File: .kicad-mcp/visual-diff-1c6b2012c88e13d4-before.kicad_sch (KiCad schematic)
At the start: 67 parts, among them J1 USB-C_PWR_IN, J2 USB-C_CPU_PROG, J3 USB-C_UART_BRIDGE, Q1 BSC010NE2LS, Q2 BSC010NE2LS, Q3 BSC010NE2LS, Q4 BSC010NE2LS, Q5 BSC010NE2LS, Q6 BSC010NE2LS, Q7 BSC010NE2LS, Q8 BSC010NE2LS, U1 RP2040, U2 W25Q16JVSSIQ, U3 ISL8117FRZ, U4 ISL8117FRZ, U5 ISL8117FRZ, U6 ISL8117FRZ

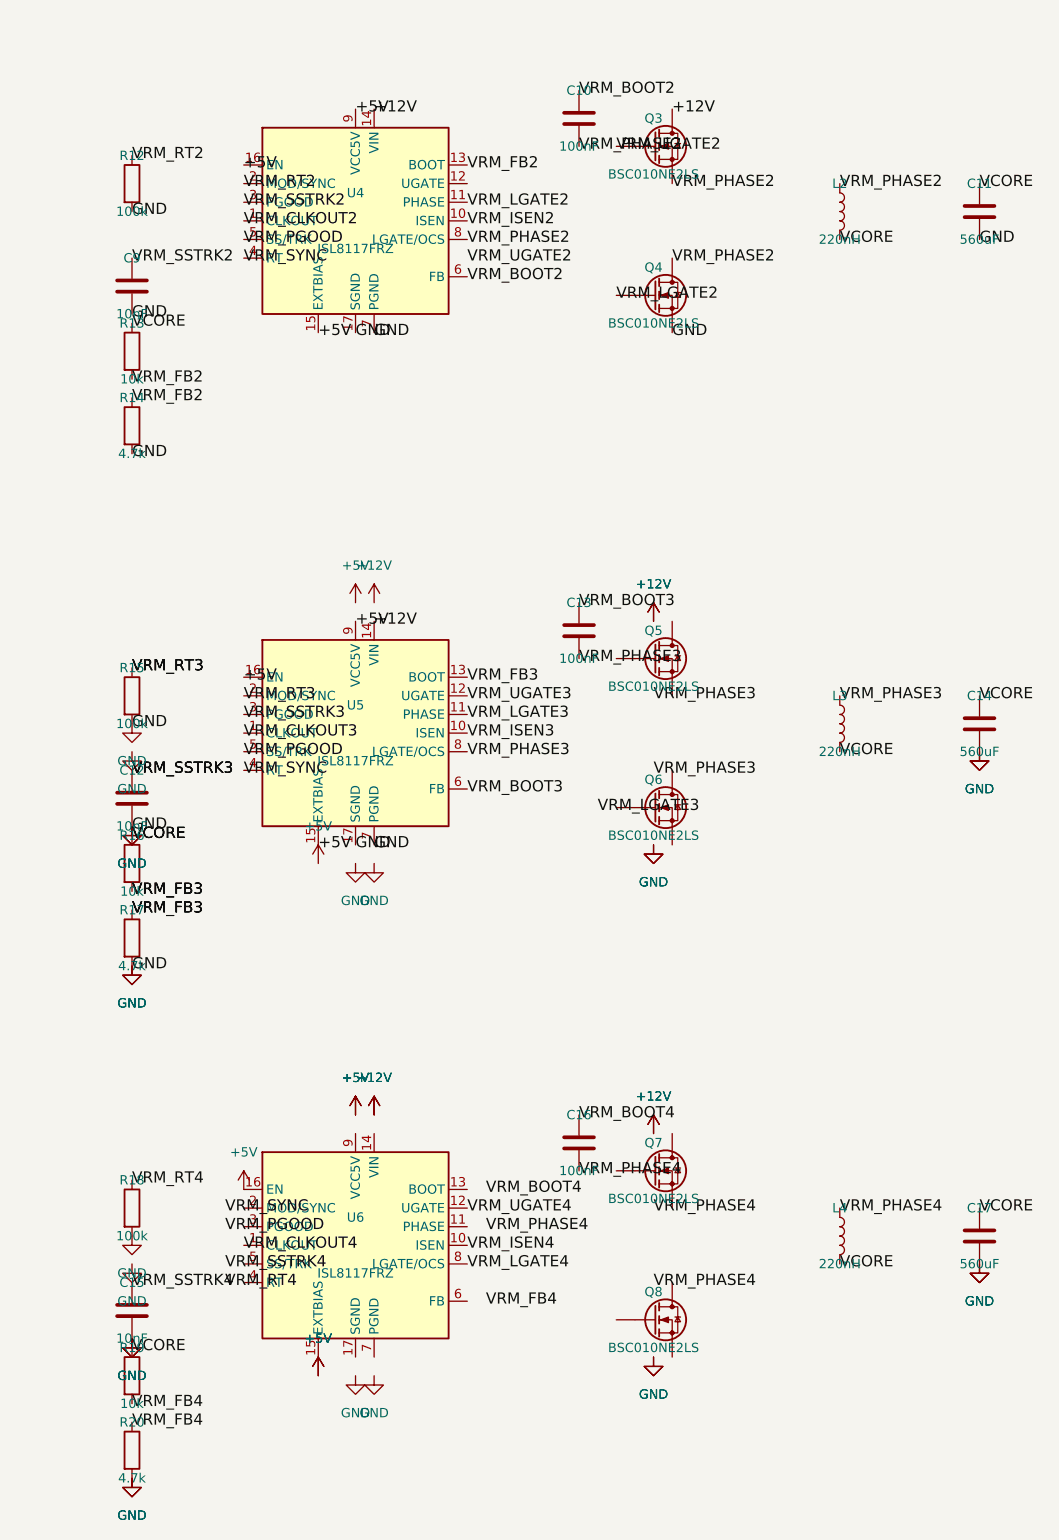
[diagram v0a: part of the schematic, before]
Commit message: Some updates1
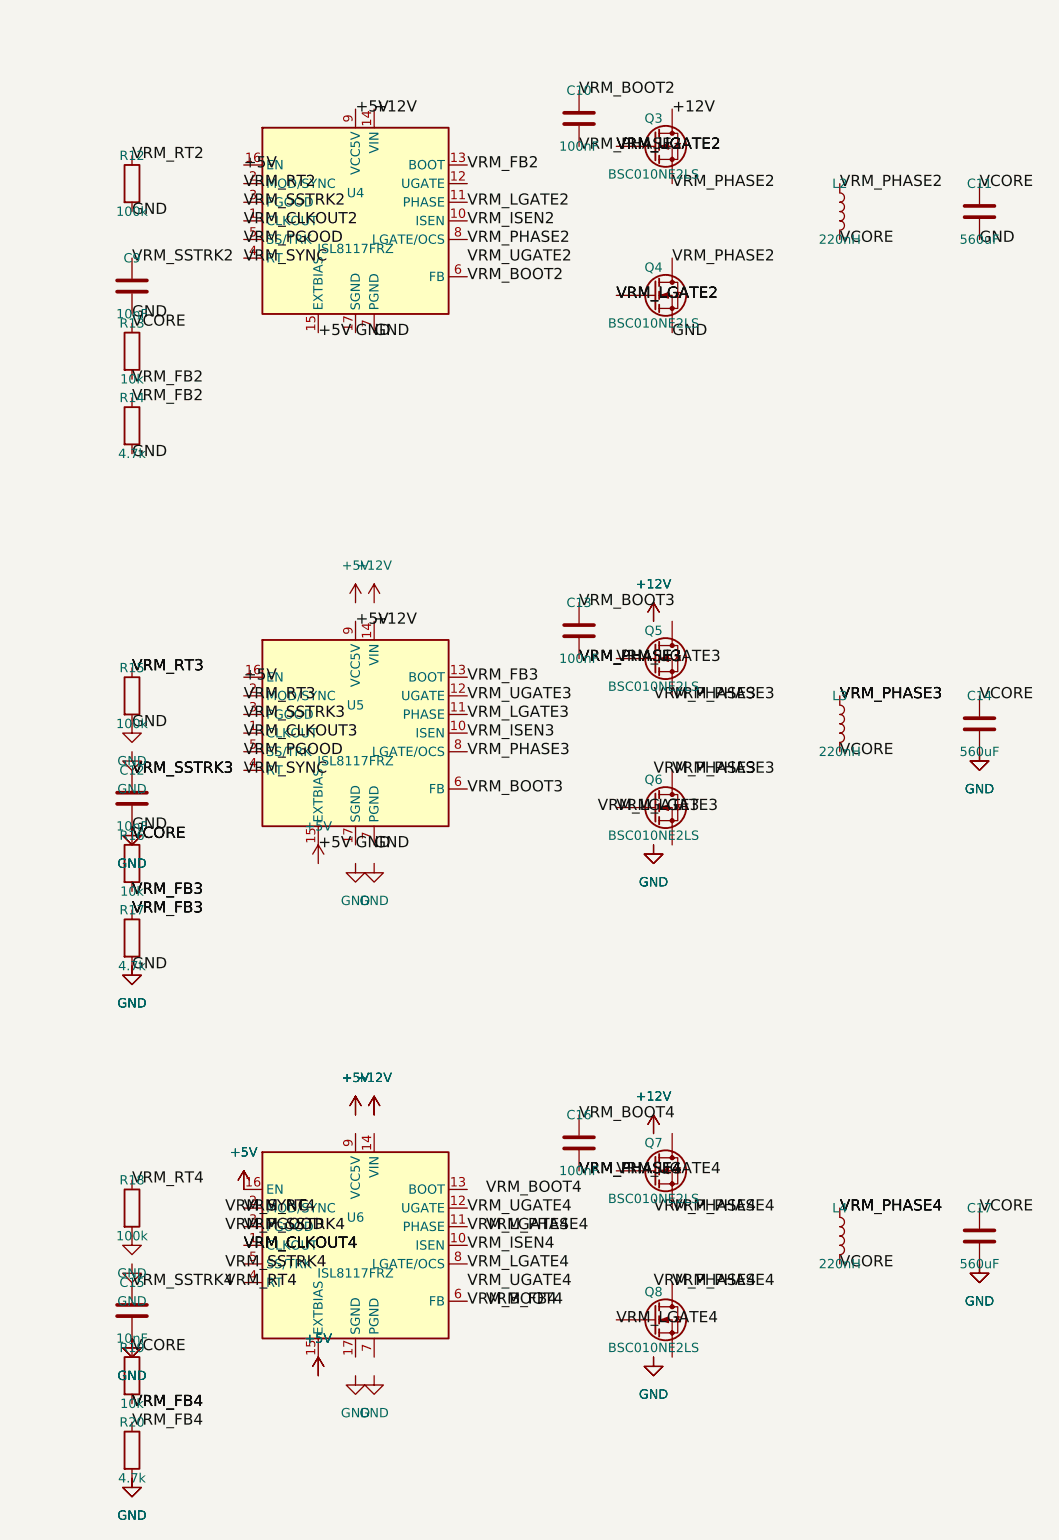
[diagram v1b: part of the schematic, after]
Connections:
- net VRM_BOOT4: now also U6.6 (FB)
- net VRM_LGATE3: now also Q6.G
- net VRM_LGATE4: now also Q8.G, U6.11 (PHASE)
- net VRM_PHASE3: now also Q5.S, Q6.D
- net VRM_PHASE4: now also Q7.S, Q8.D
- net VRM_RT4: now also U6.2 (MOD/SYNC)
- net VRM_SSTRK4: now also U6.3 (PGOOD)
- net VRM_UGATE3: now also Q5.G
- net VRM_UGATE4: now also Q7.G
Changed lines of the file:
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@@
+		(effects (font (size 1.524 1.524)))
+	)
+	(symbol
+		(lib_id "power:+5V")
+		(at 274.32 421.64 0)
+		(unit 1)
+		(exclude_from_sim no)
+		(in_bom yes)
+		(on_board yes)
+		(dnp no)
+		(property "Reference" "#PWRec1e"
+			(at 274.32 415.29 0)
+			(effects (font (size 1.27 1.27)) (hide yes))
+		)
+		(property "Value" "+5V"
+			(at 274.32 416.56 0)
+			(effects (font (size 1.27 1.27)))
+		)
+		(property "Footprint" ""
+			(at 274.32 421.64 0)
+			(effects (font (size 1.27 1.27)) (hide yes))
+		)
+		(property "Datasheet" "~"
+			(at 274.32 421.64 0)
+			(effects (font (size 1.27 1.27)) (hide yes))
+		)
+		(instances
+			(project "Ijr-X1-Core"
+				(path "/0a8e2d86-540d-4bc7-908e-89ff2a8b35b6"
+					(reference "#PWRec1e") (unit 1)
+				)
+			)
+		)
+	)
+	(label "VRM_RT4"
+		(at 274.32 424.18 0)
+		(effects (font (size 1.524 1.524)))
+	)
+	(label "VRM_SSTRK4"
+		(at 274.32 426.72 0)
+		(effects (font (size 1.524 1.524)))
+	)
+	(label "VRM_CLKOUT4"
+		(at 274.32 429.26 0)
+		(effects (font (size 1.524 1.524)))
+	)
+	(label "VRM_UGATE4"
+		(at 304.8 434.34 0)
+		(effects (font (size 1.524 1.524)))
+	)
+	(label "VRM_LGATE4"
+		(at 304.8 426.72 0)
+		(effects (font (size 1.524 1.524)))
+	)
+	(label "VRM_BOOT4"
+		(at 304.8 436.88 0)
+		(effects (font (size 1.524 1.524)))
+	)
+	(label "VRM_UGATE2"
+		(at 325.12 279.4 0)
+		(effects (font (size 1.524 1.524)))
+	)
+	(label "VRM_LGATE2"
+		(at 325.12 299.72 0)
+		(effects (font (size 1.524 1.524)))
+	)
+	(label "VRM_UGATE3"
+		(at 325.12 349.25 0)
+		(effects (font (size 1.524 1.524)))
+	)
+	(label "VRM_LGATE3"
+		(at 325.12 369.57 0)
+		(effects (font (size 1.524 1.524)))
+	)
+	(label "VRM_UGATE4"
+		(at 325.12 419.1 0)
+		(effects (font (size 1.524 1.524)))
+	)
+	(label "VRM_LGATE4"
+		(at 325.12 439.42 0)
+		(effects (font (size 1.524 1.524)))
+	)
+	(label "VRM_PHASE3"
+		(at 332.74 354.33 0)
+		(effects (font (size 1.524 1.524)))
+	)
+	(label "VRM_PHASE3"
+		(at 332.74 364.49 0)
+		(effects (font (size 1.524 1.524)))
+	)
+	(label "VRM_PHASE3"
+		(at 320.04 349.25 0)
+		(effects (font (size 1.524 1.524)))
+	)
+	(label "VRM_PHASE3"
+		(at 355.6 354.33 0)
+		(effects (font (size 1.524 1.524)))
+	)
+	(label "VRM_PHASE4"
+		(at 332.74 424.18 0)
+		(effects (font (size 1.524 1.524)))
+	)
+	(label "VRM_PHASE4"
+		(at 332.74 434.34 0)
+		(effects (font (size 1.524 1.524)))
+	)
+	(label "VRM_PHASE4"
+		(at 320.04 419.1 0)
+		(effects (font (size 1.524 1.524)))
+	)
+	(label "VRM_PHASE4"
+		(at 355.6 424.18 0)
+		(effects (font (size 1.524 1.524)))
+	)
+	(label "VRM_FB4"
+		(at 259.08 450.85 0)
 		(effects (font (size 1.524 1.524)))
 	)

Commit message: Some updates1
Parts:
- added J_DIMM1: DDR4_SO-DIMM_260, symbol dfdtc_Connector:DDR4_SODIMM_CONN260
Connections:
- net +12V: now also Q5.D, Q7.D, U6.14 (VIN)
- net +5V: now also U6.15 (EXTBIAS), U6.9 (VCC5V)
- net GND: now also Q6.S, Q8.S, U6.17 (SGND), U6.7 (PGND)
- net VRM_BOOT4: now also U6.13 (BOOT); no longer U6.6 (FB)
- net VRM_FB4: now also U6.6 (FB)
- net VRM_LGATE4: no longer U6.11 (PHASE)
- net VRM_PGOOD: now also U6.3 (PGOOD)
- net VRM_PHASE4: now also U6.11 (PHASE)
- net VRM_RT4: now also U6.4 (RT); no longer U6.2 (MOD/SYNC)
- net VRM_SSTRK4: now also U6.5 (SS/TRK); no longer U6.3 (PGOOD)
- net VRM_SYNC: now also U6.2 (MOD/SYNC)
- net VRM_UGATE2: now also U4.12 (UGATE)

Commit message: Some updates1
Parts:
- added C21, C27: 100uF, symbol Device:C
- added C22, C28: 100nF, symbol Device:C
- added C23, C24, C29, C30, C31, C32: 10uF, symbol Device:C
- added C25, C26: 47nF, symbol Device:C
- added unit 5 of J_DIMM1
- added unit 2 of J_DIMM1
- added unit 6 of J_DIMM1
- added unit 4 of J_DIMM1
- added unit 3 of J_DIMM1
- added J_DIMM2: DDR4_SO-DIMM_260, symbol dfdtc_Connector:DDR4_SODIMM_CONN260
- added J_DIMM3, J_DIMM4: DDR5_SO-DIMM_262, symbol ddr5_sodimm:DDR5_SODIMM_CONN262
- added J_M2_NVMe: M2_Key-M_NVMe, symbol Connector_Generic:Conn_02x36_Odd_Even
- added J_M2_NVMe_PCIe: M2_PCIe_Pairs, symbol Connector_Generic:Conn_01x03
- added J_PCIe_GPU_A: PCIe_x16_x8wired_pins1-41, symbol Connector_Generic:Conn_02x41_Odd_Even
- added J_PCIe_GPU_B: PCIe_x16_x8wired_pins42-82, symbol Connector_Generic:Conn_02x41_Odd_Even
- added J_RJ45: 10GBASE-T+Magnetics, symbol Connector:RJ45
- added L21: 220nH, symbol Device:L
- added L22: 1uH, symbol Device:L
- added R21, R22, R24, R28: 100k, symbol Device:R
- added R23: 316k, symbol Device:R
- added U10: AP7361C-10E, symbol Device:Regulator_Linear
- added U11: AP7361C-18E, symbol Device:Regulator_Linear
- added U7: TPS65295, symbol ti_ddr4_pwr:TPS65295
- added U9: W25Q32JV_ETH, symbol Memory_Flash:W25Q16JVSSIQ
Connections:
- net +3V3: now also C28.1, C29.1, C31.1, R28.1
- net +5V: now also U7.1 (PGOOD), U7.12 (VTTREF), U7.4 (FB_VDDQ), U7.9 (FB_VPP)
- net GND: now also J_DIMM1.1, J_DIMM1.10, J_DIMM1.14, J_DIMM1.15, J_DIMM1.18, J_DIMM1.19, J_DIMM1.2, J_DIMM1.22, J_DIMM1.23, J_DIMM1.26, J_DIMM1.27, J_DIMM1.30, J_DIMM1.31, J_DIMM1.35, J_DIMM1.36, J_DIMM1.39, J_DIMM1.40, J_DIMM1.43, J_DIMM1.44, J_DIMM1.5, J_DIMM1.6, J_DIMM1.9, C21.2, C22.2, C23.2, C24.2, C25.2, C26.2, C27.2, C28.2, C29.2, C30.2, C31.2, C32.2, J_DIMM1.102, J_DIMM1.103, J_DIMM1.106, J_DIMM1.107, J_DIMM1.167, J_DIMM1.168, J_DIMM1.171, J_DIMM1.172, J_DIMM1.175, J_DIMM1.176, J_DIMM1.180, J_DIMM1.181, J_DIMM1.184, J_DIMM1.185, J_DIMM1.188, J_DIMM1.189, J_DIMM1.192, J_DIMM1.193, J_DIMM1.196, J_DIMM1.197, J_DIMM1.201, J_DIMM1.202, J_DIMM1.205, J_DIMM1.206, J_DIMM1.209, J_DIMM1.210, J_DIMM1.213, J_DIMM1.214, J_DIMM1.217, J_DIMM1.218, J_DIMM1.222, J_DIMM1.223, J_DIMM1.226, J_DIMM1.227, J_DIMM1.230, J_DIMM1.231, J_DIMM1.234, J_DIMM1.235, J_DIMM1.238, J_DIMM1.239, J_DIMM1.243, J_DIMM1.244, J_DIMM1.247, J_DIMM1.248, J_DIMM1.251, J_DIMM1.252, J_DIMM1.47, J_DIMM1.48, J_DIMM1.51, J_DIMM1.52, J_DIMM1.56, J_DIMM1.57, J_DIMM1.60, J_DIMM1.61, J_DIMM1.64, J_DIMM1.65, J_DIMM1.68, J_DIMM1.69, J_DIMM1.72, J_DIMM1.73, J_DIMM1.77, J_DIMM1.78, J_DIMM1.81, J_DIMM1.82, J_DIMM1.85, J_DIMM1.86, J_DIMM1.89, J_DIMM1.90, J_DIMM1.93, J_DIMM1.94, J_DIMM1.98, J_DIMM1.99, J_DIMM2.1, J_DIMM2.10, J_DIMM2.102, J_DIMM2.103, J_DIMM2.106, J_DIMM2.107, J_DIMM2.14, J_DIMM2.15, J_DIMM2.167, J_DIMM2.168, J_DIMM2.171, J_DIMM2.172, J_DIMM2.175, J_DIMM2.176, J_DIMM2.18, J_DIMM2.180, J_DIMM2.181, J_DIMM2.184, J_DIMM2.185, J_DIMM2.188, J_DIMM2.189, J_DIMM2.19, J_DIMM2.192, J_DIMM2.193, J_DIMM2.196, J_DIMM2.197, J_DIMM2.2, J_DIMM2.201, J_DIMM2.202, J_DIMM2.205, J_DIMM2.206, J_DIMM2.209, J_DIMM2.210, J_DIMM2.213, J_DIMM2.214, J_DIMM2.217, J_DIMM2.218, J_DIMM2.22, J_DIMM2.222, J_DIMM2.223, J_DIMM2.226, J_DIMM2.227, J_DIMM2.23, J_DIMM2.230, J_DIMM2.231, J_DIMM2.234, J_DIMM2.235, J_DIMM2.238, J_DIMM2.239, J_DIMM2.243, J_DIMM2.244, J_DIMM2.247, J_DIMM2.248, J_DIMM2.251, J_DIMM2.252, J_DIMM2.26, J_DIMM2.27, J_DIMM2.30, J_DIMM2.31, J_DIMM2.35, J_DIMM2.36, J_DIMM2.39, J_DIMM2.40, J_DIMM2.43, J_DIMM2.44, J_DIMM2.47, J_DIMM2.48, J_DIMM2.5, J_DIMM2.51, J_DIMM2.52, J_DIMM2.56, J_DIMM2.57, J_DIMM2.6, J_DIMM2.60, J_DIMM2.61, J_DIMM2.64, J_DIMM2.65, J_DIMM2.68, J_DIMM2.69, J_DIMM2.72, J_DIMM2.73, J_DIMM2.77, J_DIMM2.78, J_DIMM2.81, J_DIMM2.82, J_DIMM2.85, J_DIMM2.86, J_DIMM2.89, J_DIMM2.9, J_DIMM2.90, J_DIMM2.93, J_DIMM2.94, J_DIMM2.98, J_DIMM2.99, R22.2, R24.2, U7.15 (GND), U7.17 (SS_VDDQ), U7.18 (SS_VPP), U7.19 (MODE)
- net DQS0_c_D1: now reaches J_DIMM1.11
- net DM0_n_DBI0_n_D1: now reaches J_DIMM1.12
- net DQS0_t_D1: now reaches J_DIMM1.13
- net DQ6_D1: now reaches J_DIMM1.16
- net DQ7_D1: now reaches J_DIMM1.17
- net DQ2_D1: now reaches J_DIMM1.20
- net DQ3_D1: now reaches J_DIMM1.21
- net DQ12_D1: now reaches J_DIMM1.24
- net DQ13_D1: now reaches J_DIMM1.25
- net DQ8_D1: now reaches J_DIMM1.28
- net DQ9_D1: now reaches J_DIMM1.29
- net DQ5_D1: now reaches J_DIMM1.3
- net DQS1_c_D1: now reaches J_DIMM1.32
- net DM1_n_DBI1_n_D1: now reaches J_DIMM1.33
- net DQS1_t_D1: now reaches J_DIMM1.34
- net DQ15_D1: now reaches J_DIMM1.37
- net DQ14_D1: now reaches J_DIMM1.38
- net DQ4_D1: now reaches J_DIMM1.4
- net DQ10_D1: now reaches J_DIMM1.41
- net DQ11_D1: now reaches J_DIMM1.42
- net DQ1_D1: now reaches J_DIMM1.7
- net DQ0_D1: now reaches J_DIMM1.8
- new net +1V0_ETH: C30.1
- new net +1V8_ETH: C32.1
- new net A0_D1: J_DIMM1.144
- new net A0_D2: J_DIMM2.144
- new net A10_AP_D1: J_DIMM1.146
- new net A10_AP_D2: J_DIMM2.146
- new net A11_D1: J_DIMM1.120
- new net A11_D2: J_DIMM2.120
- new net A12_D1: J_DIMM1.119
- new net A12_D2: J_DIMM2.119
- new net A13_D1: J_DIMM1.158
- new net A13_D2: J_DIMM2.158
- new net A1_D1: J_DIMM1.133
- new net A1_D2: J_DIMM2.133
- new net A2_D1: J_DIMM1.132
- new net A2_D2: J_DIMM2.132
- new net A3_D1: J_DIMM1.131
- new net A3_D2: J_DIMM2.131
- new net A4_D1: J_DIMM1.128
- new net A4_D2: J_DIMM2.128
- new net A5_D1: J_DIMM1.126
- new net A5_D2: J_DIMM2.126
- new net A6_D1: J_DIMM1.127
- new net A6_D2: J_DIMM2.127
- new net A7_D1: J_DIMM1.122
- new net A7_D2: J_DIMM2.122
- new net A8_D1: J_DIMM1.125
- new net A8_D2: J_DIMM2.125
- new net A9_D1: J_DIMM1.121
- new net A9_D2: J_DIMM2.121
- new net ACT_n_D1: J_DIMM1.114
- new net ACT_n_D2: J_DIMM2.114
- new net ALERT_n_D1: J_DIMM1.116
- new net ALERT_n_D2: J_DIMM2.116
- new net BA0_D1: J_DIMM1.150
- new net BA0_D2: J_DIMM2.150
- new net BA1_D1: J_DIMM1.145
- new net BA1_D2: J_DIMM2.145
- new net BG0_D1: J_DIMM1.115
- new net BG0_D2: J_DIMM2.115
- new net BG1_D1: J_DIMM1.113
- new net BG1_D2: J_DIMM2.113
- new net C0_CS2_n_NC_D1: J_DIMM1.162
- new net C0_CS2_n_NC_D2: J_DIMM2.162
- new net C1_CS3_n_NC_D1: J_DIMM1.165
- new net C1_CS3_n_NC_D2: J_DIMM2.165
- new net CAS_n_A15_D1: J_DIMM1.156
- new net CAS_n_A15_D2: J_DIMM2.156
- new net CB0_NC_D1: J_DIMM1.92
- new net CB0_NC_D2: J_DIMM2.92
- new net CB1_NC_D1: J_DIMM1.91
- new net CB1_NC_D2: J_DIMM2.91
- new net CB2_NC_D1: J_DIMM1.101
- new net CB2_NC_D2: J_DIMM2.101
- new net CB3_NC_D1: J_DIMM1.105
- new net CB3_NC_D2: J_DIMM2.105
- new net CB4_NC_D1: J_DIMM1.88
- new net CB4_NC_D2: J_DIMM2.88
- new net CB5_NC_D1: J_DIMM1.87
- new net CB5_NC_D2: J_DIMM2.87
- new net CB6_NC_D1: J_DIMM1.100
- new net CB6_NC_D2: J_DIMM2.100
- new net CB7_NC_D1: J_DIMM1.104
- new net CB7_NC_D2: J_DIMM2.104
- new net CK0_c_D1: J_DIMM1.139
- new net CK0_c_D2: J_DIMM2.139
- new net CK0_t_D1: J_DIMM1.137
- new net CK0_t_D2: J_DIMM2.137
- new net CK1_c_NF_D1: J_DIMM1.140
- new net CK1_c_NF_D2: J_DIMM2.140
- new net CK1_t_NF_D1: J_DIMM1.138
- new net CK1_t_NF_D2: J_DIMM2.138
- new net CKE0_D1: J_DIMM1.109
- new net CKE0_D2: J_DIMM2.109
- new net CKE1_NC_D1: J_DIMM1.110
- new net CKE1_NC_D2: J_DIMM2.110
- new net CS0_n_D1: J_DIMM1.149
- new net CS0_n_D2: J_DIMM2.149
- new net CS1_n_NC_D1: J_DIMM1.157
- new net CS1_n_NC_D2: J_DIMM2.157
- new net DM0_n_DBI0_n_D2: J_DIMM2.12
- new net DM1_n_DBI1_n_D2: J_DIMM2.33
- new net DM2_n_DBI2_n_D1: J_DIMM1.54
- new net DM2_n_DBI2_n_D2: J_DIMM2.54
- new net DM3_n_DBI3_n_D1: J_DIMM1.75
- new net DM3_n_DBI3_n_D2: J_DIMM2.75
- new net DM4_n_DBI4_n_D1: J_DIMM1.178
- new net DM4_n_DBI4_n_D2: J_DIMM2.178
- new net DM5_n_DBI5_n_D1: J_DIMM1.199
- new net DM5_n_DBI5_n_D2: J_DIMM2.199
- new net DM6_n_DBI6_n_D1: J_DIMM1.220
- new net DM6_n_DBI6_n_D2: J_DIMM2.220
- new net DM7_n_DBI7_n_D1: J_DIMM1.241
- new net DM7_n_DBI7_n_D2: J_DIMM2.241
- new net DM8_n_DBI_n_NC_D1: J_DIMM1.96
- new net DM8_n_DBI_n_NC_D2: J_DIMM2.96
- new net DQ0_D2: J_DIMM2.8
- new net DQ10_D2: J_DIMM2.41
- new net DQ11_D2: J_DIMM2.42
- new net DQ12_D2: J_DIMM2.24
- new net DQ13_D2: J_DIMM2.25
- new net DQ14_D2: J_DIMM2.38
- new net DQ15_D2: J_DIMM2.37
- new net DQ16_D1: J_DIMM1.50
- new net DQ16_D2: J_DIMM2.50
- new net DQ17_D1: J_DIMM1.49
- new net DQ17_D2: J_DIMM2.49
- new net DQ18_D1: J_DIMM1.62
- new net DQ18_D2: J_DIMM2.62
- new net DQ19_D1: J_DIMM1.63
- new net DQ19_D2: J_DIMM2.63
- new net DQ1_D2: J_DIMM2.7
- new net DQ20_D1: J_DIMM1.46
- new net DQ20_D2: J_DIMM2.46
- new net DQ21_D1: J_DIMM1.45
- new net DQ21_D2: J_DIMM2.45
- new net DQ22_D1: J_DIMM1.58
- new net DQ22_D2: J_DIMM2.58
- new net DQ23_D1: J_DIMM1.59
- new net DQ23_D2: J_DIMM2.59
- new net DQ24_D1: J_DIMM1.70
- new net DQ24_D2: J_DIMM2.70
- new net DQ25_D1: J_DIMM1.71
- new net DQ25_D2: J_DIMM2.71
- new net DQ26_D1: J_DIMM1.83
- new net DQ26_D2: J_DIMM2.83
- new net DQ27_D1: J_DIMM1.84
- new net DQ27_D2: J_DIMM2.84
- new net DQ28_D1: J_DIMM1.66
- new net DQ28_D2: J_DIMM2.66
- new net DQ29_D1: J_DIMM1.67
- new net DQ29_D2: J_DIMM2.67
- new net DQ2_D2: J_DIMM2.20
- new net DQ30_D1: J_DIMM1.79
- new net DQ30_D2: J_DIMM2.79
- new net DQ31_D1: J_DIMM1.80
- new net DQ31_D2: J_DIMM2.80
- new net DQ32_D1: J_DIMM1.174
- new net DQ32_D2: J_DIMM2.174
- new net DQ33_D1: J_DIMM1.173
- new net DQ33_D2: J_DIMM2.173
- new net DQ34_D1: J_DIMM1.187
- new net DQ34_D2: J_DIMM2.187
- new net DQ35_D1: J_DIMM1.186
- new net DQ35_D2: J_DIMM2.186
- new net DQ36_D1: J_DIMM1.170
- new net DQ36_D2: J_DIMM2.170
- new net DQ37_D1: J_DIMM1.169
- new net DQ37_D2: J_DIMM2.169
- new net DQ38_D1: J_DIMM1.183
- new net DQ38_D2: J_DIMM2.183
- new net DQ39_D1: J_DIMM1.182
- new net DQ39_D2: J_DIMM2.182
- new net DQ3_D2: J_DIMM2.21
- new net DQ40_D1: J_DIMM1.195
- new net DQ40_D2: J_DIMM2.195
- new net DQ41_D1: J_DIMM1.194
- new net DQ41_D2: J_DIMM2.194
- new net DQ42_D1: J_DIMM1.207
- new net DQ42_D2: J_DIMM2.207
- new net DQ43_D1: J_DIMM1.208
- new net DQ43_D2: J_DIMM2.208
- new net DQ44_D1: J_DIMM1.191
- new net DQ44_D2: J_DIMM2.191
- new net DQ45_D1: J_DIMM1.190
- new net DQ45_D2: J_DIMM2.190
- new net DQ46_D1: J_DIMM1.203
- new net DQ46_D2: J_DIMM2.203
- new net DQ47_D1: J_DIMM1.204
- new net DQ47_D2: J_DIMM2.204
- new net DQ48_D1: J_DIMM1.216
- new net DQ48_D2: J_DIMM2.216
- new net DQ49_D1: J_DIMM1.215
- new net DQ49_D2: J_DIMM2.215
- new net DQ4_D2: J_DIMM2.4
- new net DQ50_D1: J_DIMM1.228
- new net DQ50_D2: J_DIMM2.228
- new net DQ51_D1: J_DIMM1.229
- new net DQ51_D2: J_DIMM2.229
- new net DQ52_D1: J_DIMM1.211
- new net DQ52_D2: J_DIMM2.211
- new net DQ53_D1: J_DIMM1.212
- new net DQ53_D2: J_DIMM2.212
- new net DQ54_D1: J_DIMM1.224
- new net DQ54_D2: J_DIMM2.224
- new net DQ55_D1: J_DIMM1.225
- new net DQ55_D2: J_DIMM2.225
- new net DQ56_D1: J_DIMM1.237
- new net DQ56_D2: J_DIMM2.237
- new net DQ57_D1: J_DIMM1.236
- new net DQ57_D2: J_DIMM2.236
- new net DQ58_D1: J_DIMM1.249
- new net DQ58_D2: J_DIMM2.249
- new net DQ59_D1: J_DIMM1.250
- new net DQ59_D2: J_DIMM2.250
- new net DQ5_D2: J_DIMM2.3
- new net DQ60_D1: J_DIMM1.232
- new net DQ60_D2: J_DIMM2.232
- new net DQ61_D1: J_DIMM1.233
- new net DQ61_D2: J_DIMM2.233
- new net DQ62_D1: J_DIMM1.245
- new net DQ62_D2: J_DIMM2.245
- new net DQ63_D1: J_DIMM1.246
- new net DQ63_D2: J_DIMM2.246
- new net DQ6_D2: J_DIMM2.16
- new net DQ7_D2: J_DIMM2.17
- new net DQ8_D2: J_DIMM2.28
- new net DQ9_D2: J_DIMM2.29
- new net DQS0_c_D2: J_DIMM2.11
- new net DQS0_t_D2: J_DIMM2.13
- new net DQS1_c_D2: J_DIMM2.32
- new net DQS1_t_D2: J_DIMM2.34
- new net DQS2_c_D1: J_DIMM1.53
- new net DQS2_c_D2: J_DIMM2.53
- new net DQS2_t_D1: J_DIMM1.55
- new net DQS2_t_D2: J_DIMM2.55
- new net DQS3_c_D1: J_DIMM1.74
- new net DQS3_c_D2: J_DIMM2.74
- new net DQS3_t_D1: J_DIMM1.76
- new net DQS3_t_D2: J_DIMM2.76
- new net DQS4_c_D1: J_DIMM1.177
- new net DQS4_c_D2: J_DIMM2.177
- new net DQS4_t_D1: J_DIMM1.179
- new net DQS4_t_D2: J_DIMM2.179
- new net DQS5_c_D1: J_DIMM1.198
- new net DQS5_c_D2: J_DIMM2.198
- new net DQS5_t_D1: J_DIMM1.200
- new net DQS5_t_D2: J_DIMM2.200
- new net DQS6_c_D1: J_DIMM1.219
- new net DQS6_c_D2: J_DIMM2.219
- new net DQS6_t_D1: J_DIMM1.221
- new net DQS6_t_D2: J_DIMM2.221
- new net DQS7_c_D1: J_DIMM1.240
- new net DQS7_c_D2: J_DIMM2.240
- new net DQS7_t_D1: J_DIMM1.242
- new net DQS7_t_D2: J_DIMM2.242
- new net DQS8_c_D1: J_DIMM1.95
- new net DQS8_c_D2: J_DIMM2.95
- new net DQS8_t_D1: J_DIMM1.97
- new net DQS8_t_D2: J_DIMM2.97
- new net ETH_LAN_PWR_GOOD: R28.2
- new net EVENT_n_NF_D1: J_DIMM1.134
- new net EVENT_n_NF_D2: J_DIMM2.134
- new net ODT0_D1: J_DIMM1.155
- new net ODT0_D2: J_DIMM2.155
- new net ODT1_NC_D1: J_DIMM1.161
- new net ODT1_NC_D2: J_DIMM2.161
- new net PARITY_D1: J_DIMM1.143
- new net PARITY_D2: J_DIMM2.143
- new net RAS_n_A16_D1: J_DIMM1.152
- new net RAS_n_A16_D2: J_DIMM2.152
- new net RESET_n_D1: J_DIMM1.108
- new net RESET_n_D2: J_DIMM2.108
- new net SA0_D1: J_DIMM1.256
- new net SA0_D2: J_DIMM2.256
- new net SA1_D1: J_DIMM1.260
- new net SA1_D2: J_DIMM2.260
- new net SA2_D1: J_DIMM1.166
- new net SA2_D2: J_DIMM2.166
- new net SCL_SPD: J_DIMM1.253, J_DIMM2.253
- new net SDA_SPD: J_DIMM1.254, J_DIMM2.254
- new net VDDSPD_DDR4: J_DIMM1.255, J_DIMM2.255
- new net VDD_DDR4: J_DIMM1.111, J_DIMM1.112, J_DIMM1.117, J_DIMM1.118, J_DIMM1.123, J_DIMM1.124, J_DIMM1.129, J_DIMM1.130, J_DIMM1.135, J_DIMM1.136, J_DIMM1.141, J_DIMM1.142, J_DIMM1.147, J_DIMM1.148, J_DIMM1.153, J_DIMM1.154, J_DIMM1.159, J_DIMM1.160, J_DIMM1.163, J_DIMM2.111, J_DIMM2.112, J_DIMM2.117, J_DIMM2.118, J_DIMM2.123, J_DIMM2.124, J_DIMM2.129, J_DIMM2.130, J_DIMM2.135, J_DIMM2.136, J_DIMM2.141, J_DIMM2.142, J_DIMM2.147, J_DIMM2.148, J_DIMM2.153, J_DIMM2.154, J_DIMM2.159, J_DIMM2.160, J_DIMM2.163
- new net VPP_DDR4: J_DIMM1.257, J_DIMM1.259, J_DIMM2.257, J_DIMM2.259
- new net VREFCA_D1: J_DIMM1.164
- new net VREFCA_D2: J_DIMM2.164
- new net VTT_DDR4: J_DIMM1.258, J_DIMM2.258
- new net WE_n_A14_D1: J_DIMM1.151
- new net WE_n_A14_D2: J_DIMM2.151
- no-connect marks 28 -> 194
